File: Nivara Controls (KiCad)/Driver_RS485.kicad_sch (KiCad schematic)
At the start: 3 parts

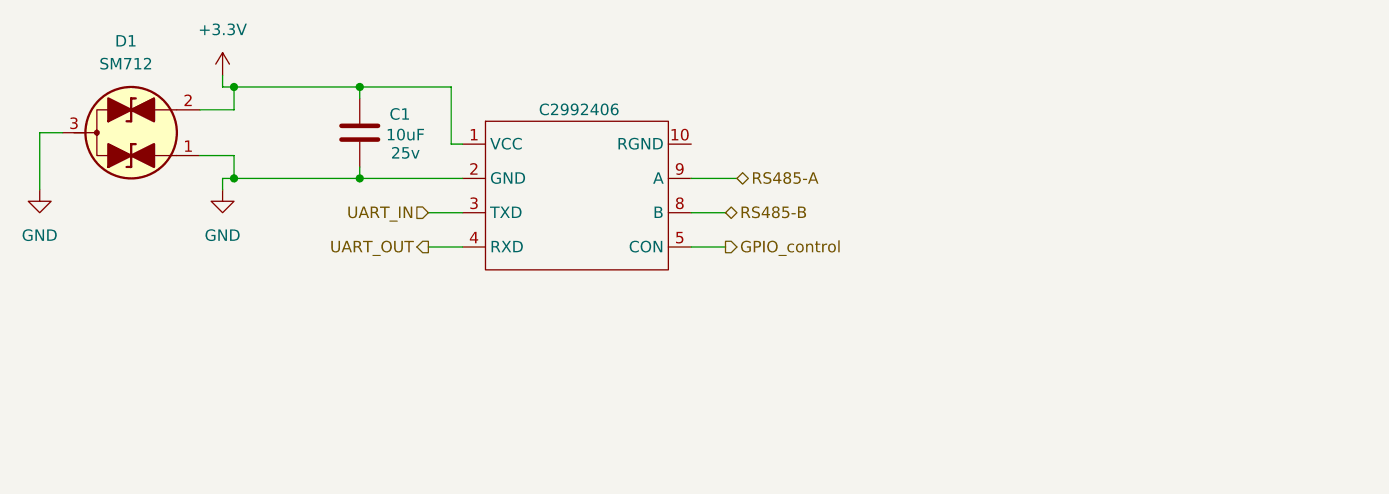
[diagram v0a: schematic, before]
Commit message: Actualización
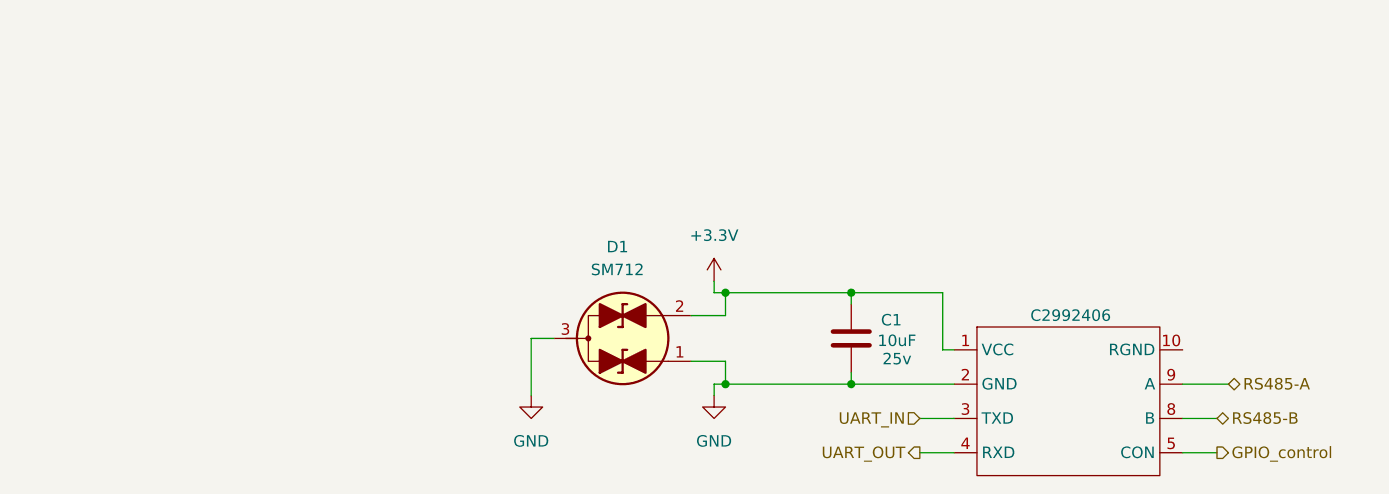
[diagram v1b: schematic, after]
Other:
- moved on the sheet: C1, C2992406, D1
